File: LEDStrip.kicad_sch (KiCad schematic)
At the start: 4 parts, among them J301 WAGO 2065-100, J302 WAGO 2065-100, J303 WAGO 2065-100, U301 74AHC1G125

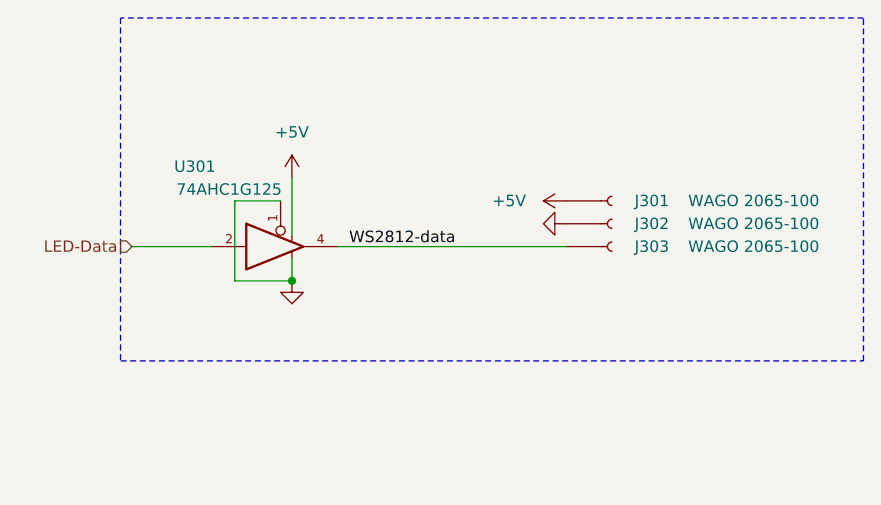
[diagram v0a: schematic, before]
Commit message: Update
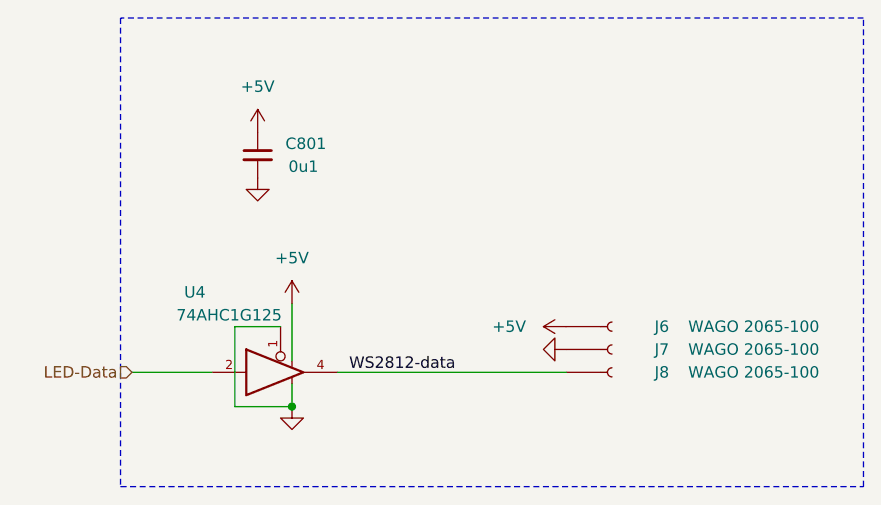
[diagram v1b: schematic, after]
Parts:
- added C801: 0u1, V2_Capacitor_SMD:C_1608, symbol V2_Capacitor:1608_0u1
- J6: renamed from J301; Id (none) -> WAGO:${SYMBOL_NAME}; Rating (none) -> 9A
- J7: renamed from J302; Id (none) -> WAGO:${SYMBOL_NAME}; Rating (none) -> 9A
- J8: renamed from J303; Id (none) -> WAGO:${SYMBOL_NAME}; Rating (none) -> 9A
- U4: renamed from U301; Id (none) -> 74xGxx:${SYMBOL_NAME}; Rating (none) -> 8mA
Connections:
- net +5V: now also C801.1
- net GND: now also C801.2
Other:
- moved on the sheet: J6, J7, J8, U4
